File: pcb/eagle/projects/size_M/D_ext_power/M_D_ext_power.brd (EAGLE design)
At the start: 21 parts

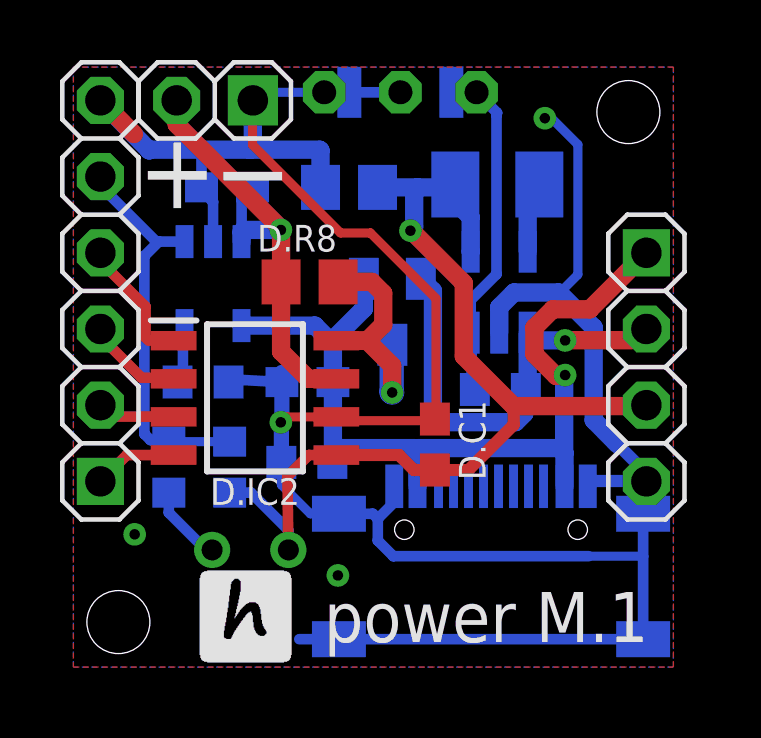
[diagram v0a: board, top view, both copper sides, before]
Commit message: PCB M.1
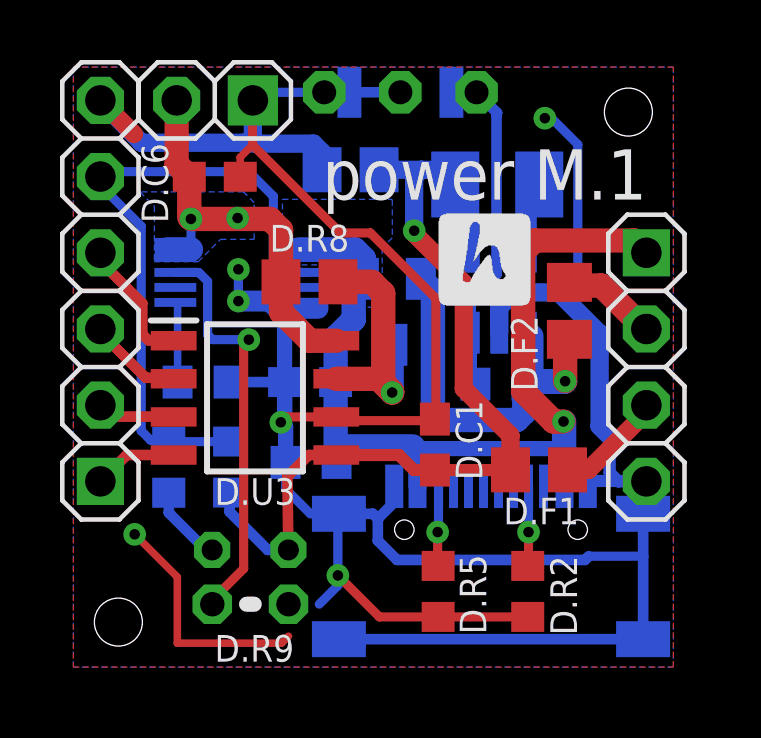
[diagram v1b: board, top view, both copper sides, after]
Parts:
- added D.F1, D.F2: (no value), rcl:R0805
- added D.R2, D.R5: 5k1, rcl:R0603
- added D.R9: TERM_10K, hugo:THERM
- D.R3: value 12k -> 1k
- D.U1: value MCP -> MCP73833-AMI_UN; device !stavebnice03:SOT23-5 -> SamacSys_Parts:SOP50P490X110-10N
- D.U2: value TC -> LM3671_3.3
- moved D.U1 1.03 mm to (6.10, 13.7), turned to 0 degrees
- moved D.C7 0.59 mm to (9.74, 17.1)
- moved D.C6 0.54 mm to (5.21, 16.8), flipped to the top
- moved D.R7 0.18 mm to (14.7, 9.93)
- moved D.R4 0.14 mm to (8.43, 7.32)
- moved D.C4 0.09 mm to (8.39, 10.0)
- renumbered D.IC2 to D.U3
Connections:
- removed net N$11: D.R3.2, D.U1.5
- removed net N$12: D.J3.2, D.R7.1, D.T1.S, D.U2.VIN
- removed net N$13: D.C6.2, D.LIPOL.2, D.R8.2, D.U1.3, D.U3.7
- removed net N$8: D.R8.1, D.T1.D, D.U3.8
- removed net N$9: D.C4.2, D.J3.1, D.R4.2, D.T1.G, D.U1.4, U$1.A4B9, U$1.B4A9
- removed net VDD: D.C1.2, D.C7.2, D.D1.2, D.J3.3, D.L1.2, D.R1.1, D.U2.BP, D.U3.5
- new net 3V3F: D.F1.2, D.J3.3
- new net IN+: D.C6.2, D.LIPOL.2, D.R8.2, D.U1.10, D.U1.9, D.U3.8
- new net IN-: D.R8.1, D.T1.D, D.U3.7
- new net N$10: D.R9.2, D.U1.8
- new net N$4: D.R5.1, U$1.B5
- new net N$6: D.R2.1, U$1.A5
- new net N$7: D.R3.2, D.U1.6
- new net VBATF: D.F2.2, D.J3.2
- new net VCC: D.C1.2, D.C7.2, D.D1.2, D.F1.1, D.L1.2, D.R1.1, D.U2.BP, D.U3.5
- new net VMOT: D.F2.1, D.R7.1, D.T1.S, D.U2.VIN
- new net VUSB: D.C4.2, D.J3.1, D.R4.2, D.T1.G, D.U1.1, D.U1.2, U$1.A4B9, U$1.B4A9
- net GND: now also D.R2.2, D.R5.2, D.R9.1, D.U1.5; no longer D.U1.2
- net P4: now also D.U1.3; no longer D.U1.1
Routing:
- net VUSB: track 0.00 -> 35.7 mm, vias 0 -> 1
- net VDD: track 34.2 -> 0.00 mm, vias 1 -> 0
- net N$9: track 33.0 -> 0.00 mm, vias 1 -> 0
- net VCC: track 0.00 -> 30.9 mm, vias 0 -> 1
- net GND: track 99.6 -> 122.1 mm, vias 4 -> 6
- net N$13: track 16.0 -> 0.00 mm, vias 1 -> 0
- net N$12: track 14.8 -> 0.00 mm, vias 1 -> 0
- net IN+: track 0.00 -> 14.8 mm, vias 0 -> 2
- net VMOT: track 0.00 -> 14.6 mm, vias 0 -> 1
- net N$10: track 0.00 -> 13.7 mm, vias 0 -> 1
- net N$8: track 9.31 -> 0.00 mm, vias 1 -> 0
- net IN-: track 0.00 -> 8.86 mm, vias 0 -> 1
- net P4: track 14.6 -> 21.8 mm
- net 3V3F: track 0.00 -> 3.66 mm
- net VBATF: track 0.00 -> 3.21 mm
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- added copper zone on layer 16, net IN+
- added copper zone on layer 16, net VUSB
